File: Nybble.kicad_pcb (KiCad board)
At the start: 2 copper layers, 106 parts, among them J1 USB_mini_micro_B, SW1 SW_PUSH, U1 ATMEGA32U4, X1 XTAL_GND

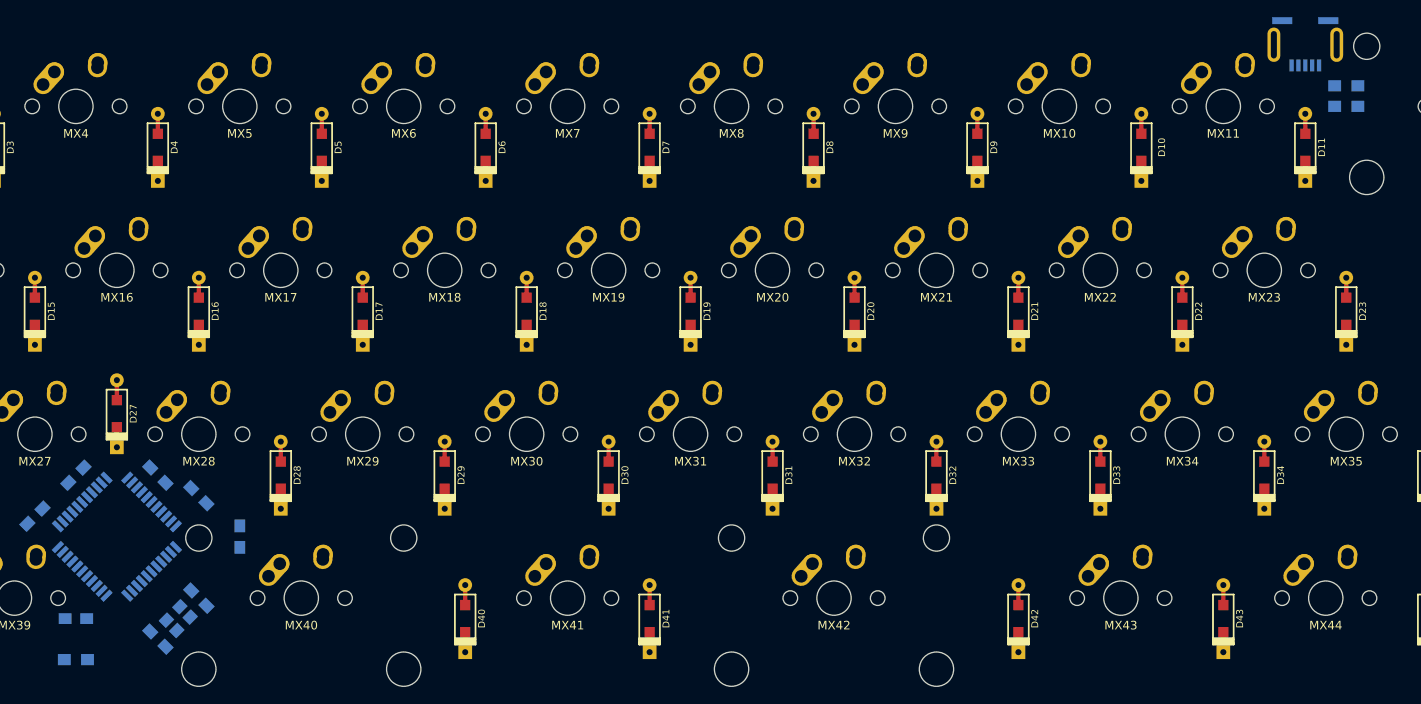
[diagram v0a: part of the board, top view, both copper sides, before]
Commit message: Made a few fine edits to the controller
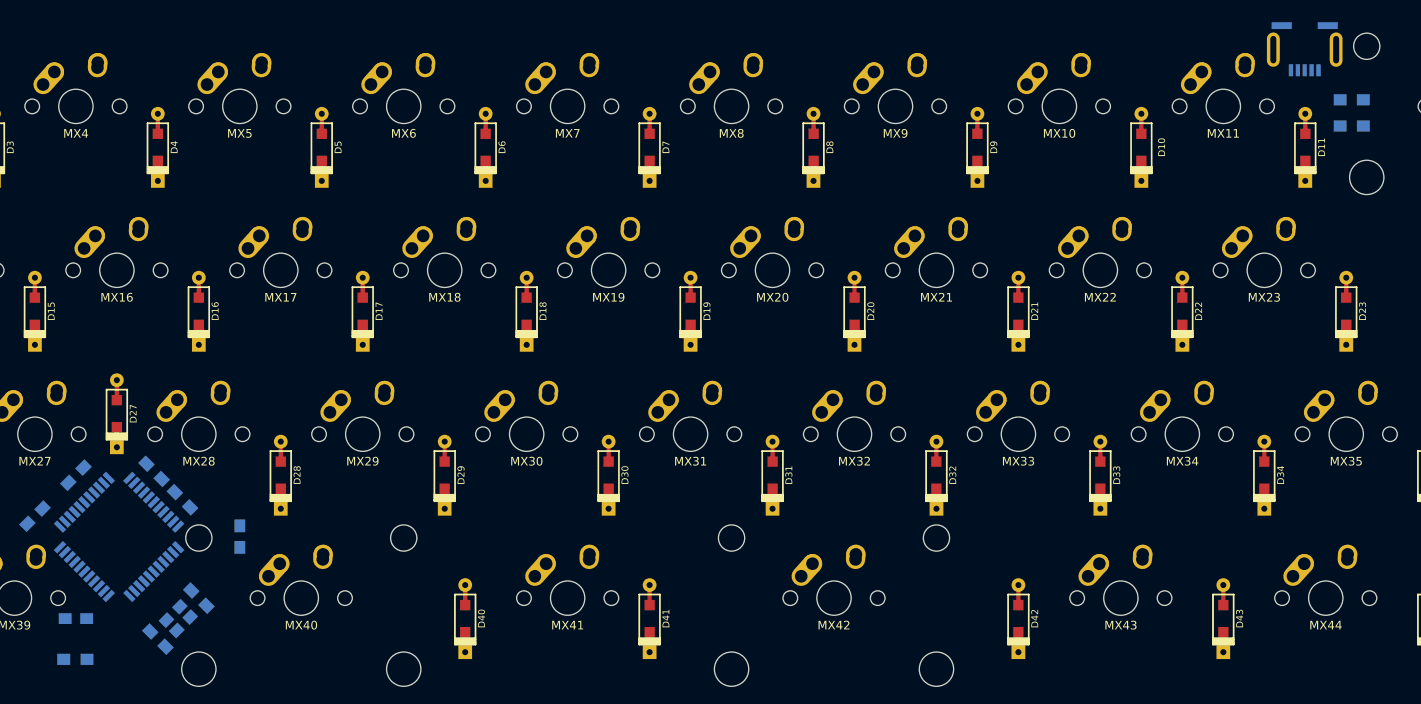
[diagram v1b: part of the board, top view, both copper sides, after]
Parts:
- moved R3 2.37 mm to (231.6, 30.9)
- moved C4 1.96 mm to (95.7, 74.3)
- moved R4 1.74 mm to (231.6, 27.8)
- moved C8 0.63 mm to (92.4, 71.0)
- moved J1 0.58 mm to (226.2, 24.4)
- moved U1 0.26 mm to (88.4, 78.6)
- moved R2 0.07 mm to (83.3, 92.8)
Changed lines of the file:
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@@
     (aux_axis_origin 0 0)
     (grid_origin 145.25625 85.725)
-    (visible_elements 7FFFE7FF)
+    (visible_elements 7FFFF7FF)
     (pcbplotparams
       (layerselection 0x00030_80000001)
@@
   )
   (module Capacitors_SMD:C_0805_HandSoldering (layer B.Cu)
-    (at 97.63125 73.81875 135)
+    (at 95.72625 74.295 135)
     (descr "Capacitor SMD 0805, hand soldering")
     (tags "capacitor 0805")
@@
   )
   (module Capacitors_SMD:C_0805_HandSoldering (layer B.Cu)
-    (at 92.86875 71.4375 135)
+    (at 92.42425 70.993 135)
     (descr "Capacitor SMD 0805, hand soldering")
     (tags "capacitor 0805")
@@
   )
   (module keyboard_parts:USB_miniB_hirose_5S8 (layer B.Cu)
-    (at 226.21875 23.8125)
+    (at 226.15525 24.384)
     (descr "USB miniB hirose UX60SC-MB-5S8")
     (tags "USB miniB hirose through hole UX60SC-MB-5S8")
@@
   )
   (module Resistors_SMD:R_0805_HandSoldering (layer B.Cu)
-    (at 83.34375 92.86875)
+    (at 83.28025 92.837)
     (descr "Resistor SMD 0805, hand soldering")
     (tags "resistor 0805")
@@
   )
   (module Resistors_SMD:R_0805_HandSoldering (layer B.Cu)
-    (at 230.98125 28.575 180)
+    (at 231.61625 30.861 180)
     (descr "Resistor SMD 0805, hand soldering")
     (tags "resistor 0805")
@@
   )
   (module Resistors_SMD:R_0805_HandSoldering (layer B.Cu)
-    (at 230.98125 26.19375 180)
+    (at 231.61625 27.813 180)
     (descr "Resistor SMD 0805, hand soldering")
     (tags "resistor 0805")
@@
   )
   (module Housings_QFP:TQFP-44_10x10mm_Pitch0.8mm (layer B.Cu)
-    (at 88.10625 78.58125 225)
+    (at 88.36025 78.613 225)
     (descr "44-Lead Plastic Thin Quad Flatpack (PT) - 10x10x1.0 mm Body [TQFP] (see Microchip Packaging Specification 00000049BS.pdf)")
     (tags "QFP 0.8")
